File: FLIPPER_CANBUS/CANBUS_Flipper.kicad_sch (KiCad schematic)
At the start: 17 parts, among them J1 Conn_01x10_Socket, J2 Conn_01x08_Socket, J3 Conn_01x02, J4 Conn_01x02_Socket, U1 MCP2515-xST, U2 MAX3051, Y1 16 Mhz

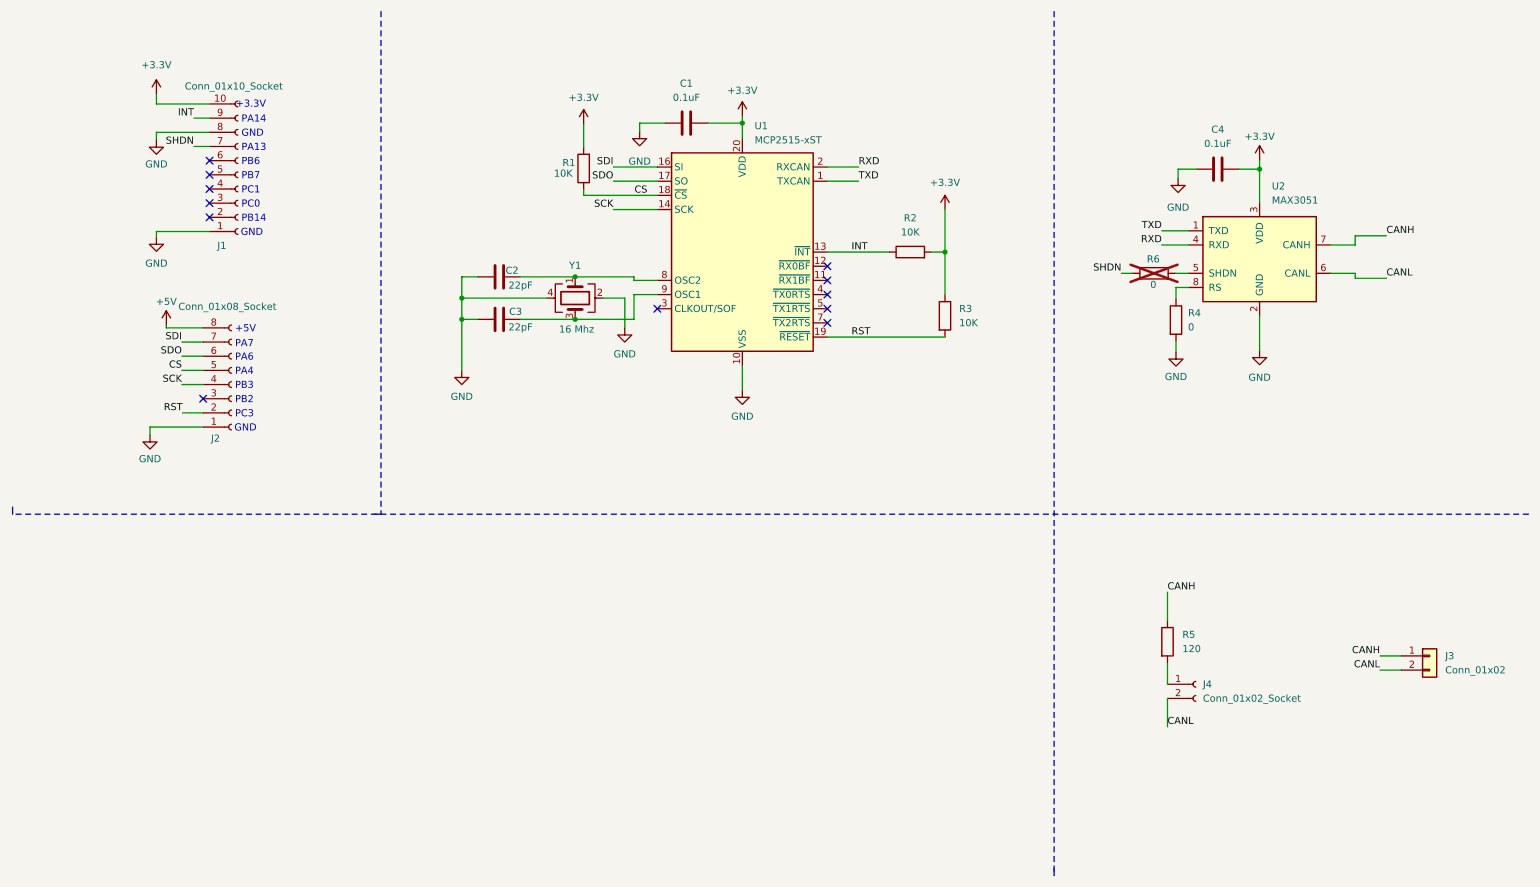
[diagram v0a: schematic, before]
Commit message: feat(Hw):Update_Schematic
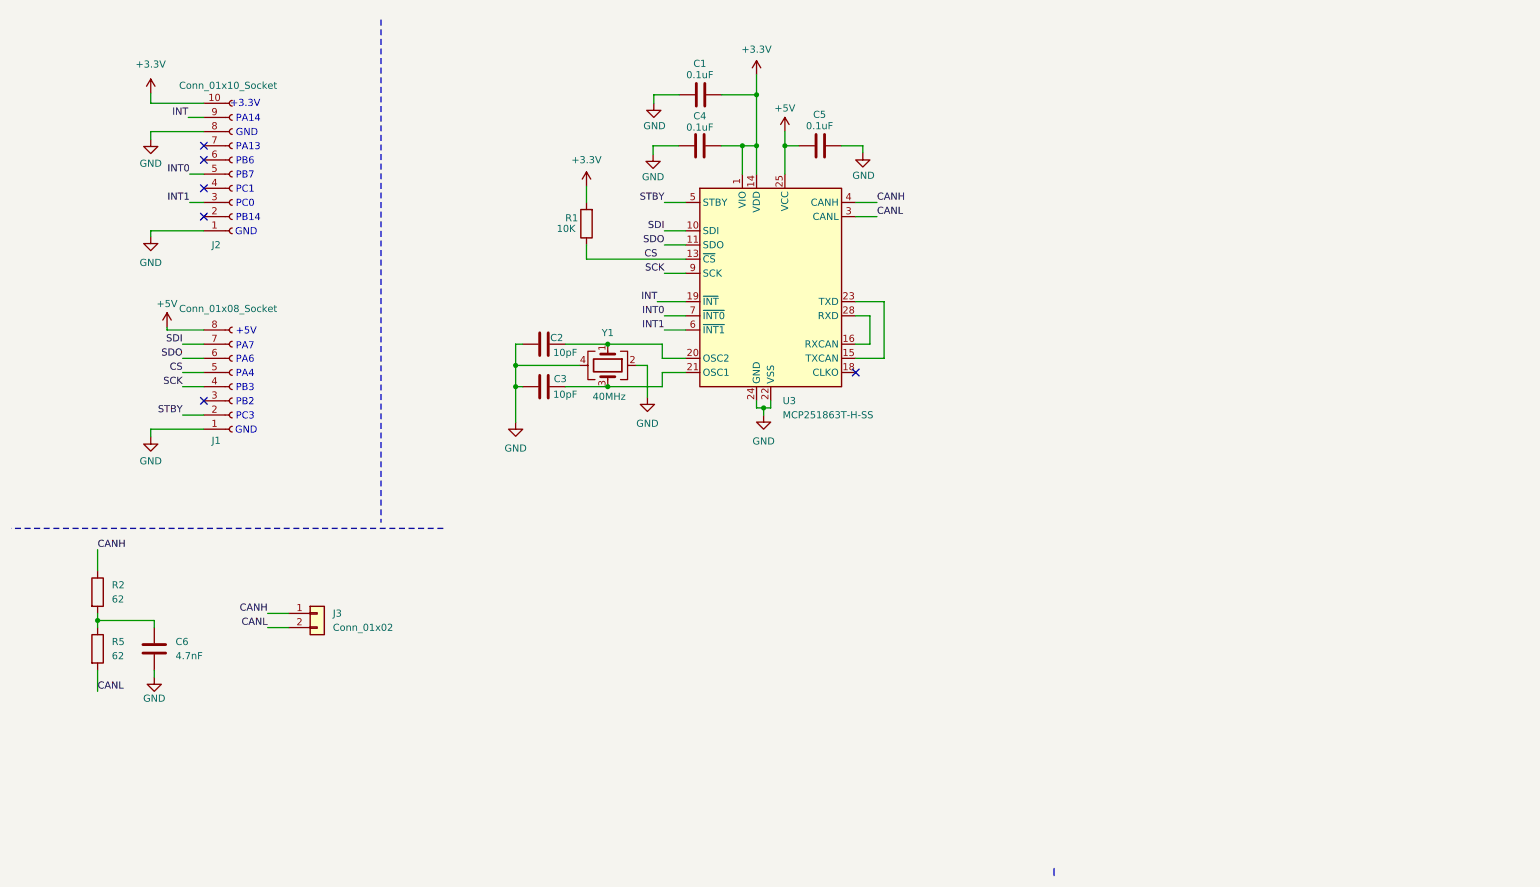
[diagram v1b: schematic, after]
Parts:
- removed J4: Conn_01x02_Socket, Connector_PinHeader_2.54mm:PinHeader_1x02_P2.54mm_Vertical, symbol Connector:Conn_01x02_Socket
- removed R3: 10K, Resistor_SMD:R_0603_1608Metric_Pad0.98x0.95mm_HandSolder, symbol Device:R
- removed R4, R6: 0, Resistor_SMD:R_0603_1608Metric_Pad0.98x0.95mm_HandSolder, symbol Device:R
- removed U1: MCP2515-xST, Package_SO:TSSOP-20_4.4x6.5mm_P0.65mm, symbol Interface_CAN_LIN:MCP2515-xST
- removed U2: MAX3051, Package_TO_SOT_SMD:SOT-23-8_Handsoldering, symbol Interface_UART:MAX3051
- added C5: 0.1uF, Capacitor_SMD:C_0603_1608Metric_Pad1.08x0.95mm_HandSolder, symbol Device:C
- added C6: 4.7nF, Capacitor_SMD:C_0603_1608Metric, symbol Device:C
- added U3: MCP251863T-H-SS, Package_SO:SSOP-28_5.3x10.2mm_P0.65mm, symbol Interface_CAN_LIN:MCP251863T-H-SS
- C2, C3: value 22pF -> 10pF; LCSC# C91701 -> C106245; manf# 0603CG220J500NT -> (none)
- R2: value 10K -> 62; LCSC# C217281 -> C351635; manf# CR-03JL7---10K -> (none)
- R5: value 120 -> 62; LCSC# C2828631 -> C351635; manf# AR03BTCX1200 -> (none)
- Y1: value 16 Mhz -> 40MHz
- renumbered J2 to J1, J1 to J2
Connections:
- net +3.3V: now also U3.1 (VIO), U3.14 (VDD); no longer R2.2
- net +5V: now also C5.1, U3.25 (VCC)
- net CANH: now also R2.1, U3.4 (CANH); no longer R5.1
- net CANL: now also R5.2, U3.3 (CANL)
- net CS: now also U3.13 (~{CS})
- net GND: now also C5.2, C6.2, U3.22 (VSS), U3.24 (GND)
- net INT: now also U3.19 (~{INT}); no longer R2.1
- net SCK: now also U3.9 (SCK)
- net SDI: now also U3.10 (SDI)
- net SDO: now also U3.11 (SDO)
- net at C2.2, Y1.1: now also U3.20 (OSC2)
- net at C3.2, Y1.3: now also U3.21 (OSC1)
- net INT1: now reaches J2.3 (Pin_3)
- net INT1: now also U3.6 (~{INT1})
- net INT0: now reaches J2.5 (Pin_5)
- net INT0: now also U3.7 (~{INT0})
- net RST renamed STBY
- net STBY: now also U3.5 (STBY)
- net SHDN: no longer names the net of J2.7 (Pin_7)
- new net: U3.15 (TXCAN), U3.23 (TXD)
- new net: U3.16 (RXCAN), U3.28 (RXD)
- new net: C6.1, R2.2, R5.1
- no-connect marks 12 -> 6
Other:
- moved on the sheet: C1, C2, C3, J2, J3, R1, R5, Y1

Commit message: feat(Hw):Update_Schematic
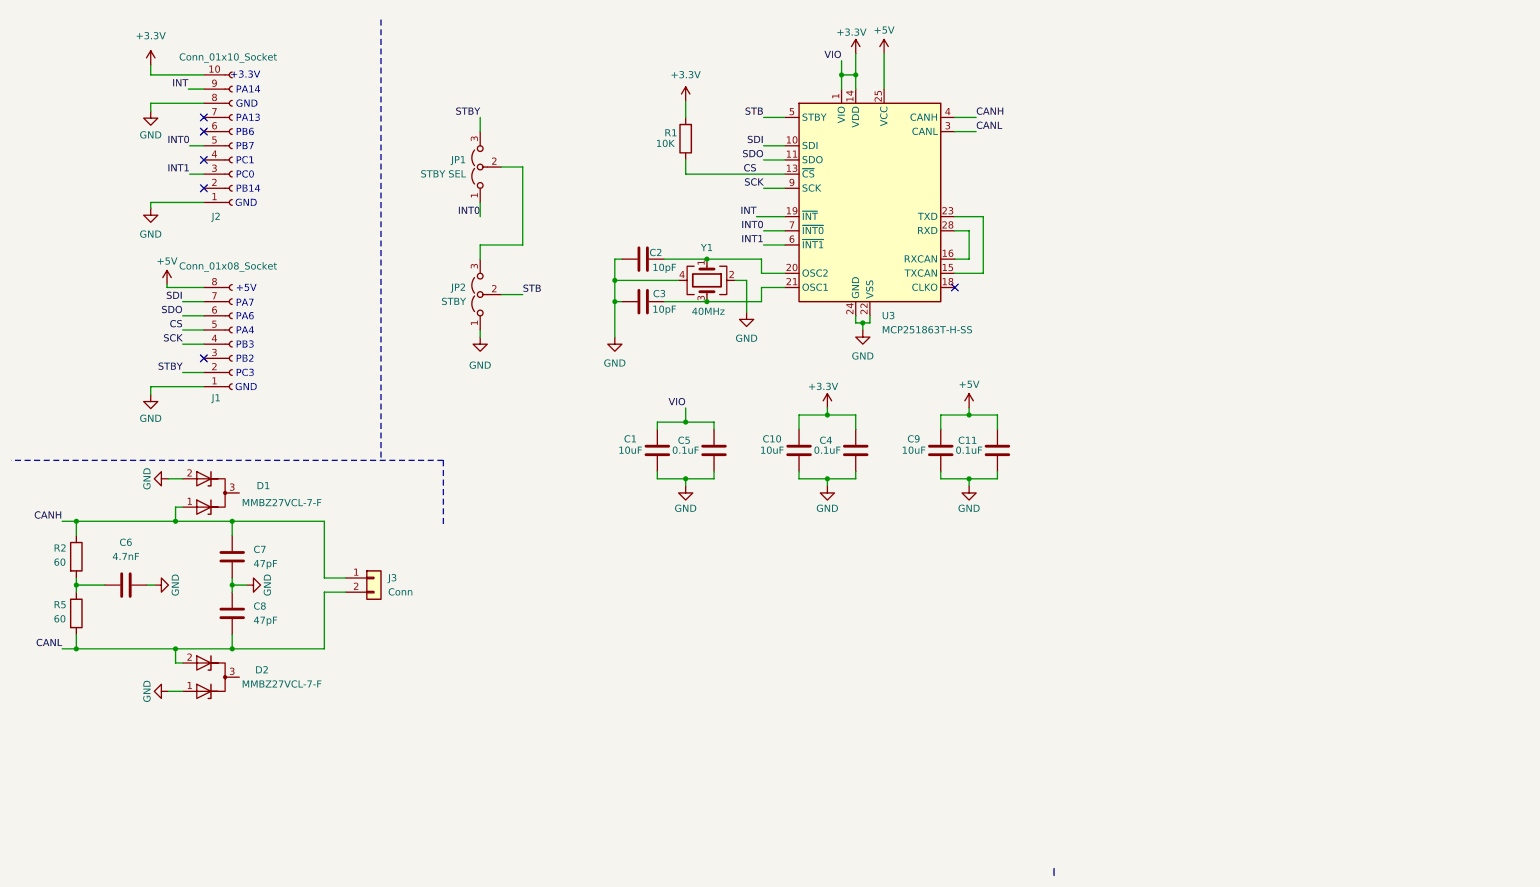
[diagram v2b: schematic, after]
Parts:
- added C10, C9: 10uF, Capacitor_SMD:C_0603_1608Metric, symbol Device:C
- added C11: 0.1uF, Capacitor_SMD:C_0603_1608Metric_Pad1.08x0.95mm_HandSolder, symbol Device:C
- added C7, C8: 47pF, Capacitor_SMD:C_0603_1608Metric, symbol Device:C
- added D1, D2: MMBZ27VCL-7-F, Package_TO_SOT_SMD:SOT-23, symbol Diode:MMBZxx
- added JP1: STBY SEL, symbol Jumper:Jumper_3_Open
- added JP2: STBY, symbol Jumper:Jumper_3_Open
- C1: value 0.1uF -> 10uF; footprint Capacitor_SMD:C_0603_1608Metric_Pad1.08x0.95mm_HandSolder -> Capacitor_SMD:C_0603_1608Metric; LCSC# C14663 -> C19702; Manufactura LCSC -> (none); manf# CC0603KRX7R9BB104 -> (none)
- C4, C5: manf# CC0603KRX7R9BB104 -> (none)
- J1: manf# PH2.54-01-08PZD -> (none)
- J2: manf# DS1021-1x10SF11-B -> (none)
- J3: value Conn_01x02 -> Conn; manf# TRT-02 -> (none)
- R1: manf# CR-03JL7---10K -> (none)
- R2, R5: value 62 -> 60; LCSC# C351635 -> C166918
- U3: LCSC# (none) -> C5226885
- Y1: LCSC# C254270 -> (none); manf# X2C016000B91H-R -> (none)
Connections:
- net +3.3V: now also C5.2, C10.2
- net +5V: now also C11.2, C9.2; no longer C5.1
- net CANH: now also C7.2, D1.1 (K)
- net CANL: now also C8.1, D2.2 (K)
- net GND: now also C5.1, C10.1, C11.1, C7.1, C8.2, C9.1, D1.2 (K), D2.1 (K), JP2.1 (A); no longer C5.2
- net INT0: now also JP1.1 (A)
- net STBY: now also JP1.3 (B); no longer U3.5 (STBY)
- new net: JP1.2 (C), JP2.3 (B)
- new net STB: JP2.2 (C), U3.5 (STBY)
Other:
- moved on the sheet: C2, C3, C4, C6, J1, J2, J3, R1, R2, R5, U3, Y1
